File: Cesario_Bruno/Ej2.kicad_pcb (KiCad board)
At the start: 2 copper layers, 16 parts, among them P1 CONN_01X14, P2 CONN_01X14, U1 SN74LVC1GX04, U2 74HCT4053, U3 LTC5507, X1 XTAL

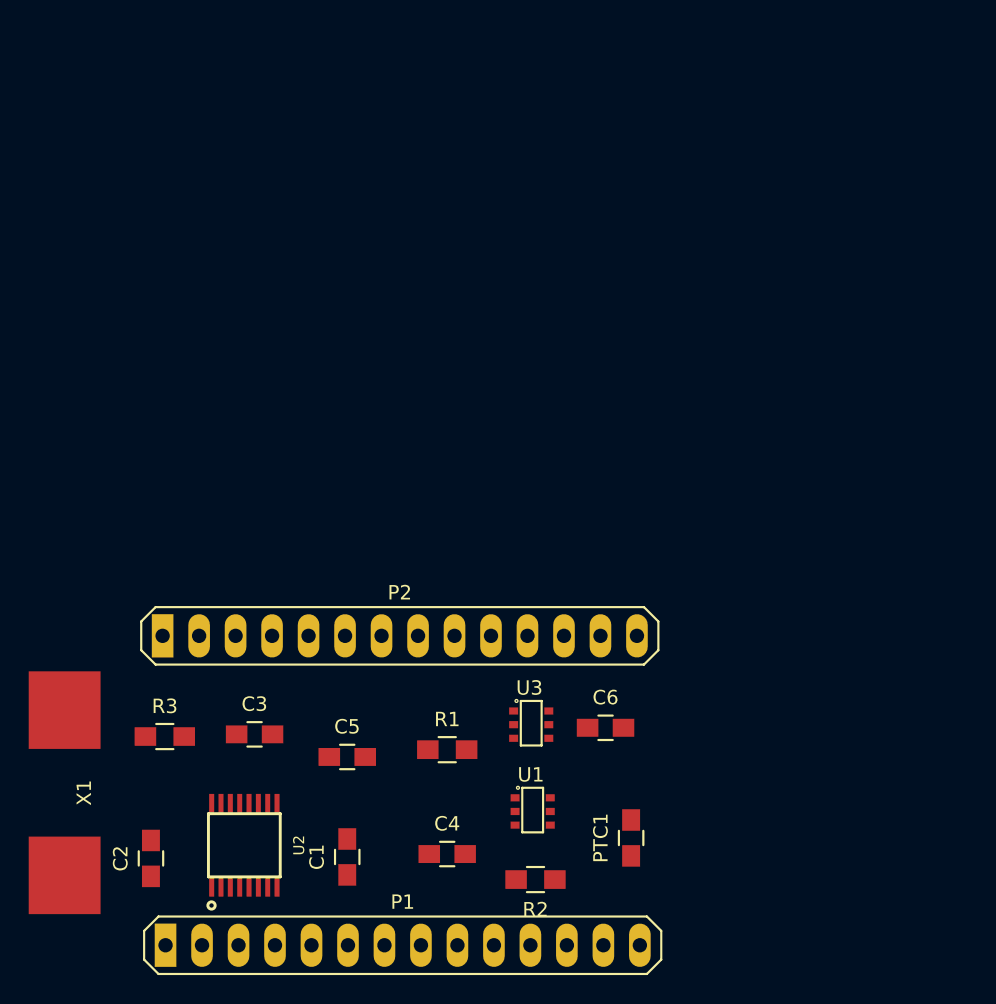
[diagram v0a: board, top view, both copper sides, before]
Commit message: Prueba de Ruteo PCB ambas capas. Finalizado.
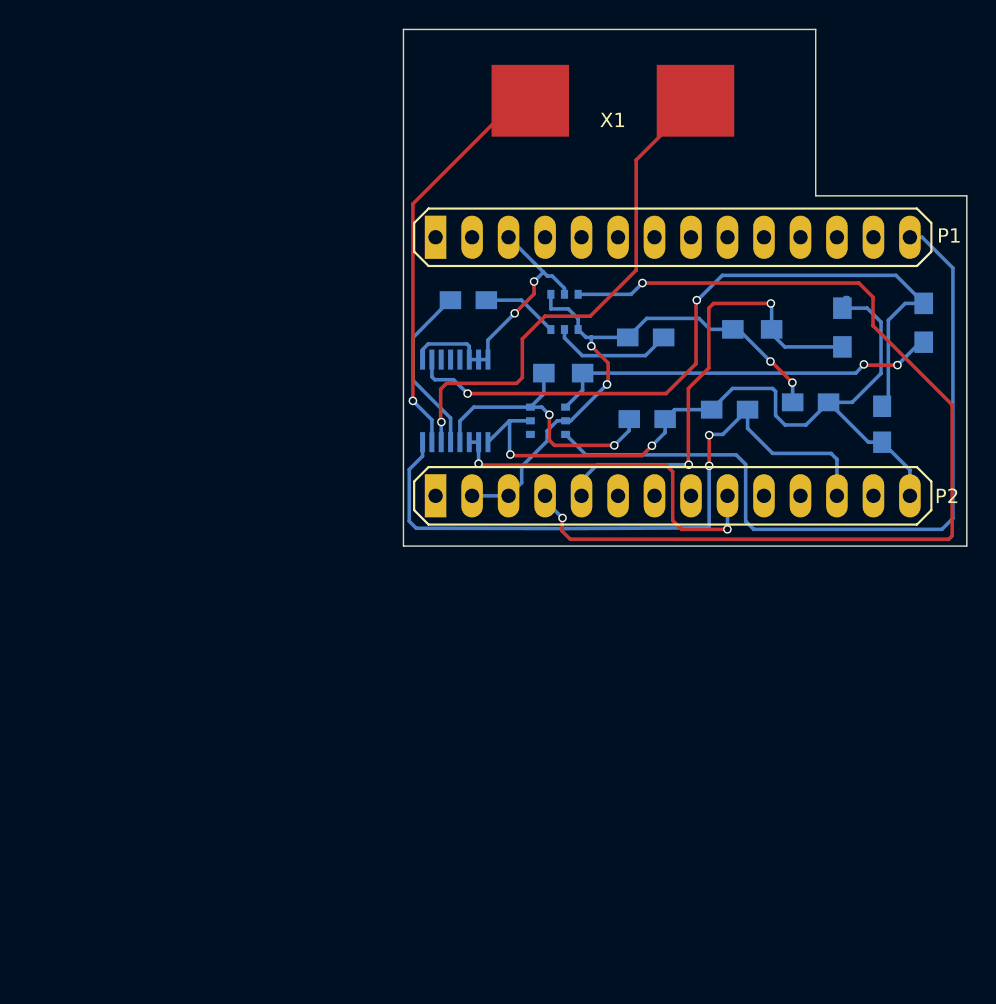
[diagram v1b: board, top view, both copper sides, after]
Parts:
- C1, C2, C3, C4, C5, C6, R1, R2, R3, U1, U2, U3: moved to B.Cu
- PTC1: footprint Ej2:C_0805_HandSoldering -> Ej2:R_0805_HandSoldering; moved to B.Cu
- moved X1 60.9 mm to (163.8, 70.9), turned to 0 degrees
- moved R3 60.2 mm to (185.5, 86.0), turned to 270 degrees
- moved C2 59.2 mm to (182.6, 93.0), turned to 270 degrees
- moved P1 52.8 mm to (168.0, 80.0)
- moved C3 45.1 mm to (177.6, 91.5)
- moved C4 38.6 mm to (153.8, 84.4)
- moved PTC1 38.5 mm to (179.8, 86.3)
- moved C1 36.9 mm to (166.2, 92.7), turned to 180 degrees
- moved R1 36.2 mm to (173.5, 86.4)
- moved C5 35.8 mm to (166.1, 87.0)
- moved R2 35.3 mm to (160.4, 89.5)
- moved U2 34.2 mm to (152.9, 91.4), turned to 270 degrees
- moved U3 29.1 mm to (159.5, 84.0), turned to 270 degrees
- moved U1 25.3 mm to (158.1, 93.7)
- moved C6 23.8 mm to (172.0, 92.0), turned to 180 degrees
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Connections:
- PTC1 pad 1: (no net) -> /ArduinoCon/PTC
- PTC1 pad 2: (no net) -> GND
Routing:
- net GND: track 0.00 -> 74.0 mm, vias 0 -> 4
- net /ArduinoCon/ENVELOPE_IN: track 0.00 -> 70.6 mm, vias 0 -> 2
- net /ArduinoCon/FREQUENCY_IN: track 0.00 -> 53.6 mm
- net /OSC_DRIVER/Switch_IN-: track 0.00 -> 51.8 mm, vias 0 -> 2
- net +5V: track 0.00 -> 47.8 mm, vias 0 -> 2
- net +3V3: track 0.00 -> 40.4 mm, vias 0 -> 4
- net /SWITCH_ENVELOPE/xtal_N: track 0.00 -> 38.3 mm, vias 0 -> 1
- net /ArduinoCon/PTC: track 0.00 -> 32.4 mm, vias 0 -> 2
- net /SWITCH_ENVELOPE/xtal_P: track 0.00 -> 28.4 mm, vias 0 -> 1
- net Net-(R2-Pad1): track 0.00 -> 27.6 mm, vias 0 -> 2
- net /ArduinoCon/DIG_CONTROL: track 0.00 -> 25.7 mm, vias 0 -> 2
- net /OSC_DRIVER/Switch_IN+: track 0.00 -> 19.8 mm, vias 0 -> 2
- net Net-(C4-Pad1): track 0.00 -> 12.0 mm
- net Net-(C5-Pad2): track 0.00 -> 8.52 mm
- net Net-(C4-Pad2): track 0.00 -> 5.34 mm
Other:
- board outline added: 39.2 x 36 mm
